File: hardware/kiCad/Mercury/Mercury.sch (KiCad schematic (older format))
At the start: 75 parts, among them J1 SWD, J10 OUTPUT, J11 Analog I/O, J12 Power Rails, J2 UART1, J3 I2C2, J4 UART1, J5 SPI1, J6 SPI2, J7 629105150521, J8 Battery Input, J9 INPUT, Q1 AO3401A, SW1 SW_SPDT, U1 STM32F407VGT6, U2 AMS1117-3.3, U3 AMS1117-5.0, Y1 HSE 16MHz

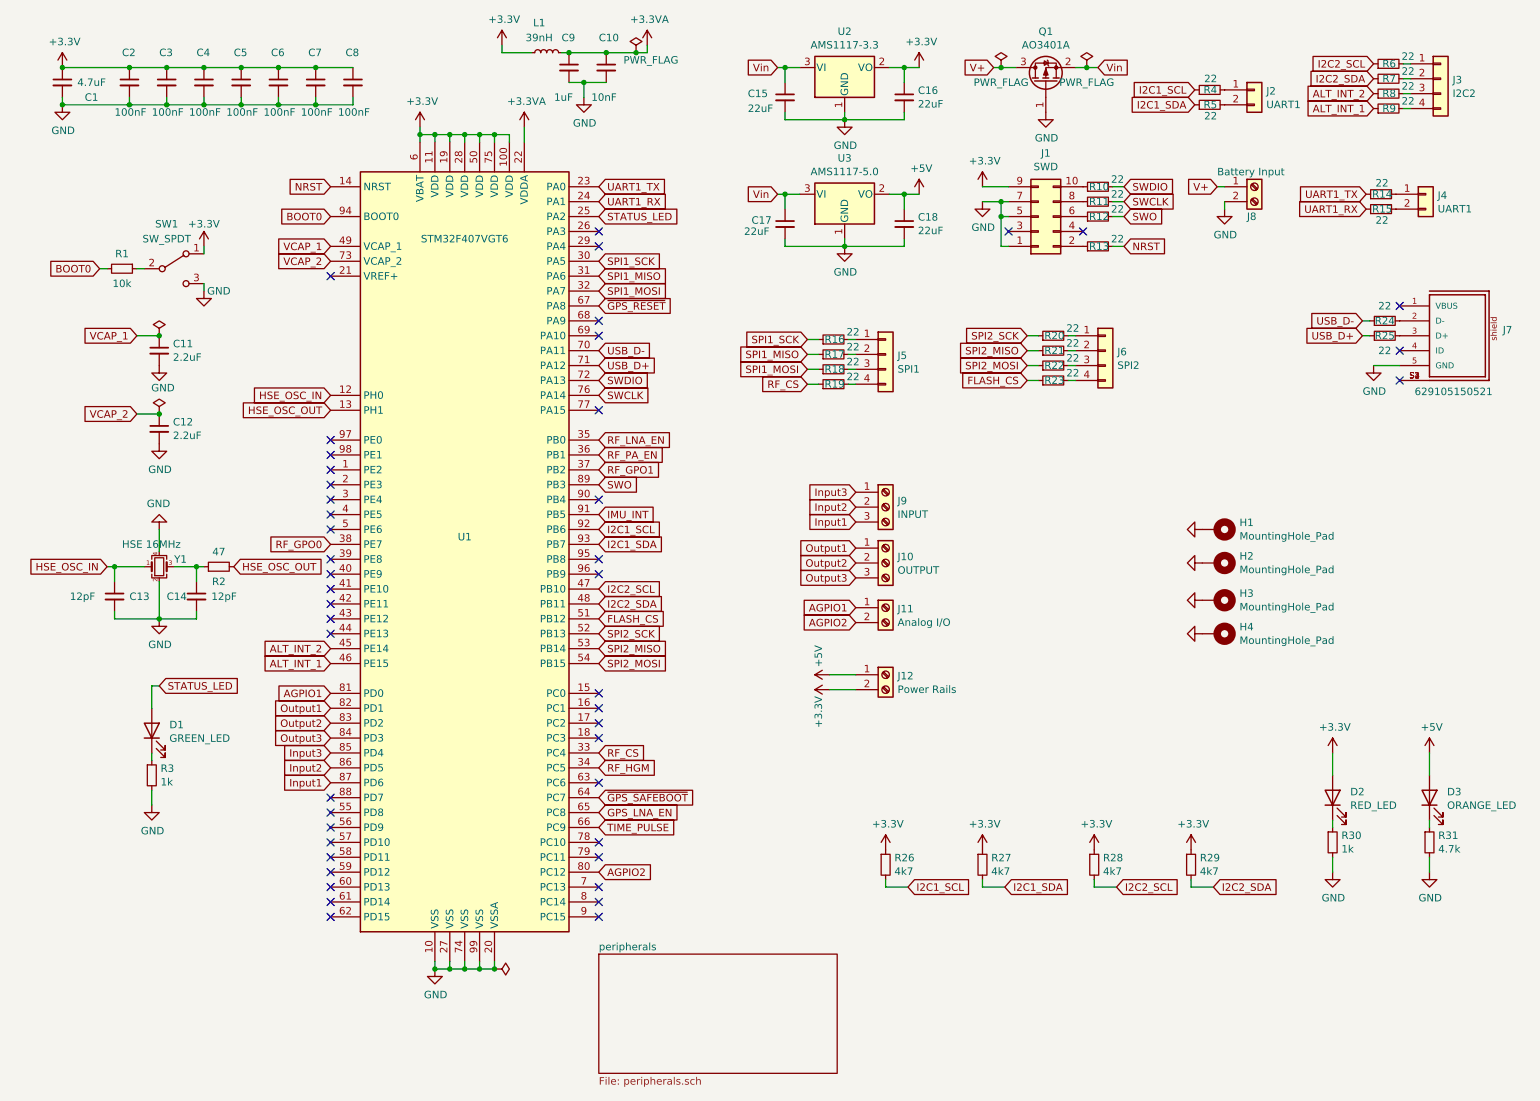
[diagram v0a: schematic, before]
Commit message: Refresh
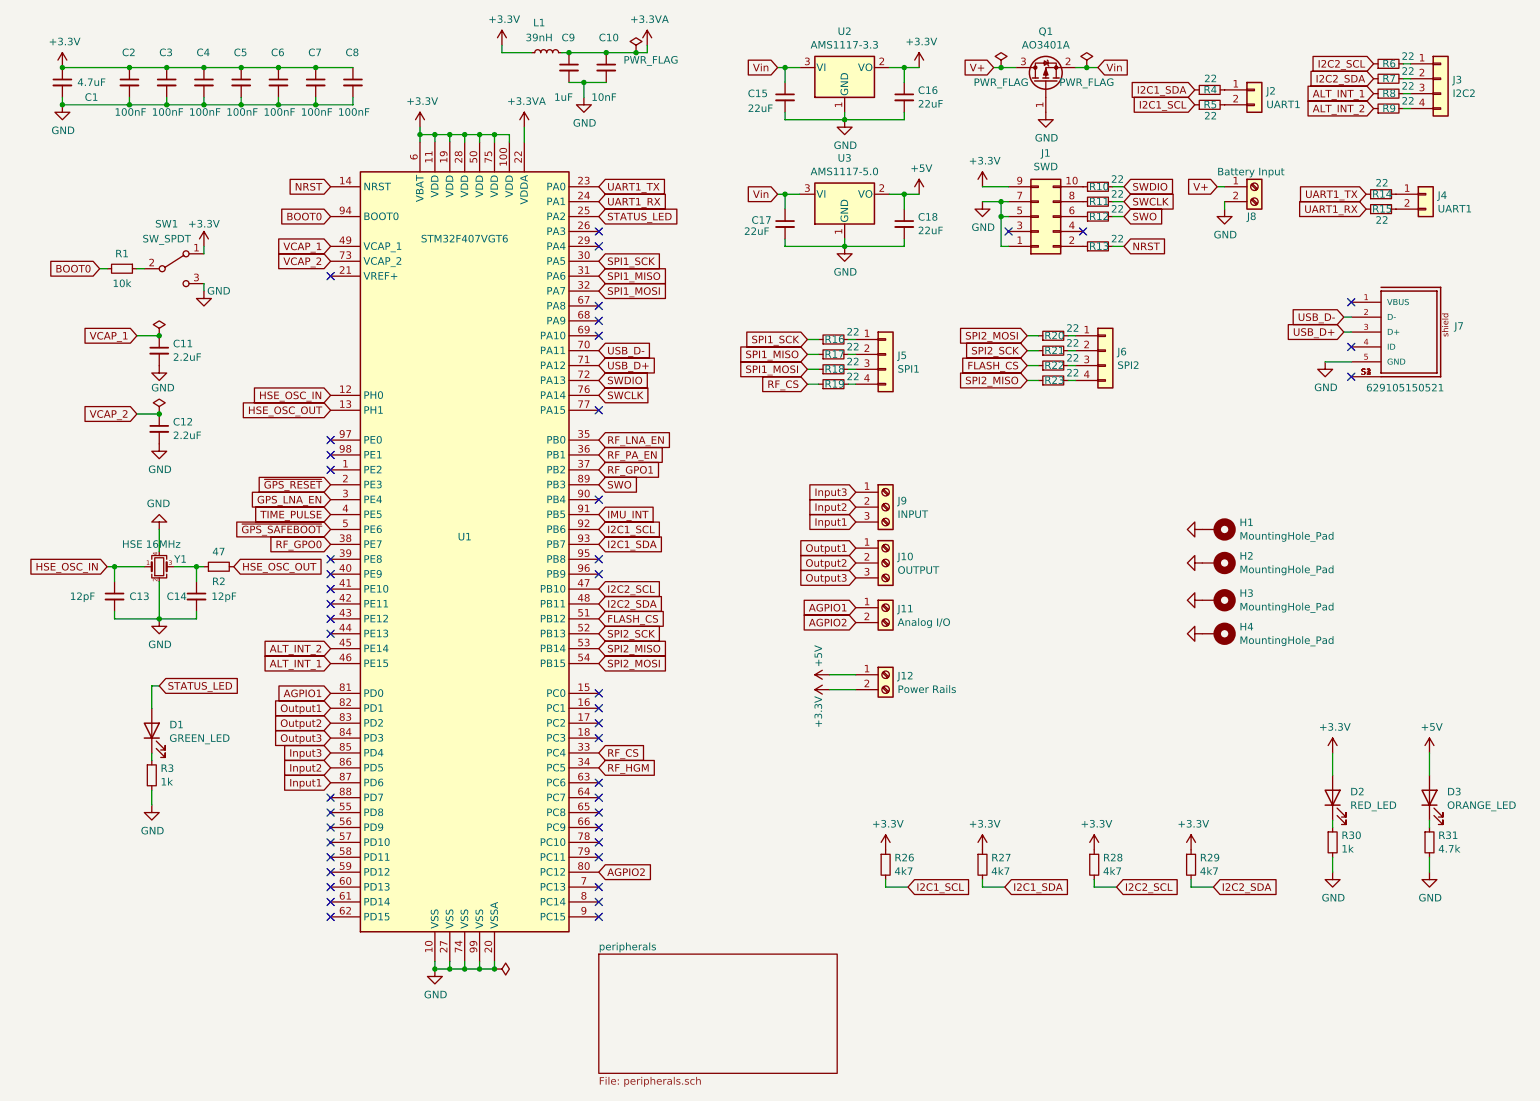
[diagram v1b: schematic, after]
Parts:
- removed R24, R25: 22, Resistor_SMD:R_0402_1005Metric, symbol Device:R_Small
- H1, H2, H3, H4: footprint MountingHole:MountingHole_4.3mm_M4_Pad_Via -> MountingHole:MountingHole_3mm_Pad_Via
- J3: footprint Connector_Wire:SolderWire-0.1sqmm_1x04_P3.6mm_D0.4mm_OD1mm_Relief -> Connector_Wire:SolderWire-0.1sqmm_1x04_P3.6mm_D0.4mm_OD1mm
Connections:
- net ALT_INT_1: now also R8.1; no longer R9.1
- net ALT_INT_2: now also R9.1; no longer R8.1
- net FLASH_CS: now also R22.1; no longer R23.1
- net GPS_LNA_EN: now also U1.3 (PE4); no longer U1.65 (PC8)
- net I2C1_SCL: now also R5.1; no longer R4.1
- net I2C1_SDA: now also R4.1; no longer R5.1
- net SPI2_MISO: now also R23.1; no longer R21.1
- net SPI2_MOSI: now also R20.1; no longer R22.1
- net SPI2_SCK: now also R21.1; no longer R20.1
- net TIME_PULSE: now also U1.4 (PE5); no longer U1.66 (PC9)
- net USB_D+: now also J7.3 (D+)
- net USB_D-: now also J7.2 (D-)
- net ~GPS_RESET: now also U1.2 (PE3); no longer U1.67 (PA8)
- net ~GPS_SAFEBOOT: now also U1.5 (PE6); no longer U1.64 (PC7)
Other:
- moved on the sheet: J7
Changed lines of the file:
@@
 Wire Wire Line
 	5550 1000 5550 1100
+Text GLabel 8300 1250 0    50   Input ~ 0
+I2C1_SCL
 Text GLabel 8300 1150 0    50   Input ~ 0
-I2C1_SCL
-Text GLabel 8300 1250 0    50   Input ~ 0
 I2C1_SDA
 Text GLabel 9500 975  0    50   Input ~ 0
@@
 	1    0    0    -1
 $EndComp
-NoConn ~ 9675 2900
-Wire Wire Line
-	9475 2700 9425 2700
-Wire Wire Line
-	9475 2800 9425 2800
-$Comp
-L Device:R_Small R24
-U 1 1 5FE85A1A
-P 9575 2700
-F 0 "R24" V 9575 2700 50  0000 C CNN
-F 1 "22" V 9675 2700 50  0000 C CNN
-F 2 "Resistor_SMD:R_0402_1005Metric" H 9575 2700 50  0001 C CNN
-F 3 "~" H 9575 2700 50  0001 C CNN
-	1    9575 2700
-	0    -1   -1   0
-$EndComp
-$Comp
-L Device:R_Small R25
-U 1 1 5FE850CF
-P 9575 2800
-F 0 "R25" V 9575 2800 50  0000 C CNN
-F 1 "22" V 9475 2800 50  0000 C CNN
-F 2 "Resistor_SMD:R_0402_1005Metric" H 9575 2800 50  0001 C CNN
-F 3 "~" H 9575 2800 50  0001 C CNN
-	1    9575 2800
-	0    -1   -1   0
-$EndComp
-NoConn ~ 9675 2600
-Text GLabel 9425 2800 0    50   Input ~ 0
+NoConn ~ 9350 2875
+Wire Wire Line
+	9350 2675 9300 2675
+Wire Wire Line
+	9350 2775 9300 2775
+NoConn ~ 9350 2575
+Text GLabel 9300 2775 0    50   Input ~ 0
 USB_D+
-Text GLabel 9425 2700 0    50   Input ~ 0
+Text GLabel 9300 2675 0    50   Input ~ 0
 USB_D-
 $Comp
 L power:GND #PWR0138
 U 1 1 5FE68EC5
-P 9500 3000
-F 0 "#PWR0138" H 9500 2750 50  0001 C CNN
-F 1 "GND" H 9505 2827 50  0000 C CNN
-F 2 "" H 9500 3000 50  0001 C CNN
-F 3 "" H 9500 3000 50  0001 C CNN
-	1    9500 3000
+P 9175 2975
+F 0 "#PWR0138" H 9175 2725 50  0001 C CNN
+F 1 "GND" H 9180 2802 50  0000 C CNN
+F 2 "" H 9175 2975 50  0001 C CNN
+F 3 "" H 9175 2975 50  0001 C CNN
+	1    9175 2975
 	1    0    0    -1
 $EndComp
@@
 Text GLabel 2500 5000 0    50   Input ~ 0
 ALT_INT_1
-Text GLabel 4300 2600 2    50   Input ~ 0
+Text GLabel 2500 3800 0    50   Input ~ 0
 ~GPS_RESET
-Text GLabel 4300 6100 2    50   Input ~ 0
+Text GLabel 2500 4000 0    50   Input ~ 0
 TIME_PULSE
-Text GLabel 4300 6000 2    50   Input ~ 0
+Text GLabel 2500 3900 0    50   Input ~ 0
 GPS_LNA_EN
 Text GLabel 4300 5600 2    50   Input ~ 0
@@
 Wire Wire Line
 	9700 1175 9750 1175
+Text GLabel 9500 1275 0    50   Input ~ 0
+ALT_INT_2
 Text GLabel 9500 1175 0    50   Input ~ 0
-ALT_INT_2
-Text GLabel 9500 1275 0    50   Input ~ 0
 ALT_INT_1
 $Comp
@@
 Wire Wire Line
 	7450 3000 7500 3000
+Text GLabel 7175 2900 0    50   Input ~ 0
+SPI2_SCK
+Wire Wire Line
+	7175 2800 7250 2800
+Text GLabel 7175 3100 0    50   Input ~ 0
+SPI2_MISO
+Wire Wire Line
+	7175 2900 7250 2900
 Text GLabel 7175 2800 0    50   Input ~ 0
-SPI2_SCK
-Wire Wire Line
-	7175 2800 7250 2800
-Text GLabel 7175 2900 0    50   Input ~ 0
-SPI2_MISO
-Wire Wire Line
-	7175 2900 7250 2900
+SPI2_MOSI
+Wire Wire Line
+	7175 3000 7250 3000
+Wire Wire Line
+	7175 3100 7250 3100
 Text GLabel 7175 3000 0    50   Input ~ 0
-SPI2_MOSI
-Wire Wire Line
-	7175 3000 7250 3000
-Wire Wire Line
-	7175 3100 7250 3100
-Text GLabel 7175 3100 0    50   Input ~ 0
 FLASH_CS
 Text GLabel 2500 5800 0    50   Input ~ 0
@@
 NoConn ~ 2500 3600
 NoConn ~ 2500 3700
-NoConn ~ 2500 3800
-NoConn ~ 2500 3900
-NoConn ~ 2500 4000
-NoConn ~ 2500 4100
+NoConn ~ 4300 5900
 NoConn ~ 2500 4300
 NoConn ~ 2500 4400
@@
 Wire Wire Line
 	7575 1000 7500 1000
-Text GLabel 4300 5900 2    50   Input ~ 0
+Text GLabel 2500 4100 0    50   Input ~ 0
 ~GPS_SAFEBOOT
 $Comp
@@
 F 0 "H1" V 8404 4250 50  0000 L CNN
 F 1 "MountingHole_Pad" V 8495 4250 50  0000 L CNN
-F 2 "MountingHole:MountingHole_4.3mm_M4_Pad_Via" H 8450 4100 50  0001 C CNN
+F 2 "MountingHole:MountingHole_3mm_Pad_Via" H 8450 4100 50  0001 C CNN
 F 3 "~" H 8450 4100 50  0001 C CNN
 	1    8450 4100
@@
 F 0 "H2" V 8404 4475 50  0000 L CNN
 F 1 "MountingHole_Pad" V 8495 4475 50  0000 L CNN
-F 2 "MountingHole:MountingHole_4.3mm_M4_Pad_Via" H 8450 4325 50  0001 C CNN
+F 2 "MountingHole:MountingHole_3mm_Pad_Via" H 8450 4325 50  0001 C CNN
 F 3 "~" H 8450 4325 50  0001 C CNN
 	1    8450 4325
@@
 F 0 "H3" V 8404 4725 50  0000 L CNN
 F 1 "MountingHole_Pad" V 8495 4725 50  0000 L CNN
-F 2 "MountingHole:MountingHole_4.3mm_M4_Pad_Via" H 8450 4575 50  0001 C CNN
+F 2 "MountingHole:MountingHole_3mm_Pad_Via" H 8450 4575 50  0001 C CNN
 F 3 "~" H 8450 4575 50  0001 C CNN
 	1    8450 4575
@@
 F 0 "H4" V 8404 4950 50  0000 L CNN
 F 1 "MountingHole_Pad" V 8495 4950 50  0000 L CNN
-F 2 "MountingHole:MountingHole_4.3mm_M4_Pad_Via" H 8450 4800 50  0001 C CNN
+F 2 "MountingHole:MountingHole_3mm_Pad_Via" H 8450 4800 50  0001 C CNN
 F 3 "~" H 8450 4800 50  0001 C CNN
 	1    8450 4800
@@
 L 629105150521:629105150521 J7
 U 1 1 5FF1E6CB
-P 10075 2800
-F 0 "J7" H 10367 2839 50  0000 L CNN
-F 1 "629105150521" H 9775 2425 50  0000 L CNN
-F 2 "629105150521:629105150521" H 10075 2800 50  0001 L BNN
-F 3 "" H 10075 2800 50  0001 L BNN
-F 4 "629105150521" H 10075 2800 50  0001 L BNN "VALUE"
-F 5 "5" H 10075 2800 50  0001 L BNN "PINS"
-F 6 "Type B" H 10075 2800 50  0001 L BNN "INTERFACE-TYPE"
-F 7 "Horizontal" H 10075 2800 50  0001 L BNN "TYPE"
-F 8 "Receptacle" H 10075 2800 50  0001 L BNN "GERDER"
-F 9 "SMT" H 10075 2800 50  0001 L BNN "MOUNT"
-F 10 "30V(AC)" H 10075 2800 50  0001 L BNN "WORKING-VOLTAGE"
-F 11 "Tape and Reel" H 10075 2800 50  0001 L BNN "PACKAGING"
-F 12 "3.0A" H 10075 2800 50  0001 L BNN "IR1"
-F 13 "629105150521" H 10075 2800 50  0001 L BNN "PART-NUMBER"
-F 14 "https://www.we-online.com/catalog/datasheet/629105150521.pdf" H 10075 2800 50  0001 L BNN "DATASHEET-URL"
-F 15 "Micro USB 2.0" H 10075 2800 50  0001 L BNN "APPLICATION"
-	1    10075 2800
-	1    0    0    -1
-$EndComp
-Wire Wire Line
-	9500 3000 9675 3000
+P 9750 2775
+F 0 "J7" H 10042 2814 50  0000 L CNN
+F 1 "629105150521" H 9450 2400 50  0000 L CNN
+F 2 "629105150521:629105150521" H 9750 2775 50  0001 L BNN
+F 3 "" H 9750 2775 50  0001 L BNN
+F 4 "629105150521" H 9750 2775 50  0001 L BNN "VALUE"
+F 5 "5" H 9750 2775 50  0001 L BNN "PINS"
+F 6 "Type B" H 9750 2775 50  0001 L BNN "INTERFACE-TYPE"
+F 7 "Horizontal" H 9750 2775 50  0001 L BNN "TYPE"
+F 8 "Receptacle" H 9750 2775 50  0001 L BNN "GERDER"
+F 9 "SMT" H 9750 2775 50  0001 L BNN "MOUNT"
+F 10 "30V(AC)" H 9750 2775 50  0001 L BNN "WORKING-VOLTAGE"
+F 11 "Tape and Reel" H 9750 2775 50  0001 L BNN "PACKAGING"
+F 12 "3.0A" H 9750 2775 50  0001 L BNN "IR1"
+F 13 "629105150521" H 9750 2775 50  0001 L BNN "PART-NUMBER"
+F 14 "https://www.we-online.com/catalog/datasheet/629105150521.pdf" H 9750 2775 50  0001 L BNN "DATASHEET-URL"
+F 15 "Micro USB 2.0" H 9750 2775 50  0001 L BNN "APPLICATION"
+	1    9750 2775
+	1    0    0    -1
+$EndComp
+Wire Wire Line
+	9175 2975 9350 2975
 $Comp
 L power:PWR_FLAG #FLG0104
@@
 $EndComp
 Connection ~ 3600 7050
-NoConn ~ 9675 3100
+NoConn ~ 9350 3075
 NoConn ~ 4300 2700
 NoConn ~ 4300 2800
@@
 F 0 "J3" H 10030 1067 50  0000 L CNN
 F 1 "I2C2" H 10030 976 50  0000 L CNN
-F 2 "Connector_Wire:SolderWire-0.1sqmm_1x04_P3.6mm_D0.4mm_OD1mm_Relief" H 9950 1075 50  0001 C CNN
+F 2 "Connector_Wire:SolderWire-0.1sqmm_1x04_P3.6mm_D0.4mm_OD1mm" H 9950 1075 50  0001 C CNN
 F 3 "~" H 9950 1075 50  0001 C CNN
 	1    9950 1075
 	1    0    0    -1
 $EndComp
+NoConn ~ 4300 6000
+NoConn ~ 4300 6100
+NoConn ~ 4300 2600
 $EndSCHEMATC
